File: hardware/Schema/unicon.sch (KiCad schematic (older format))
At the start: 57 parts, among them J1 PROG, J2 PWR, J3 SIDE A, J4 SIDE B, U1 LM340MP-5.0, U2 SIP21106-3.3, U3 STM32F051C8Tx, U4 AT24C16, Y1 8MHz, Y2 32768 Hz

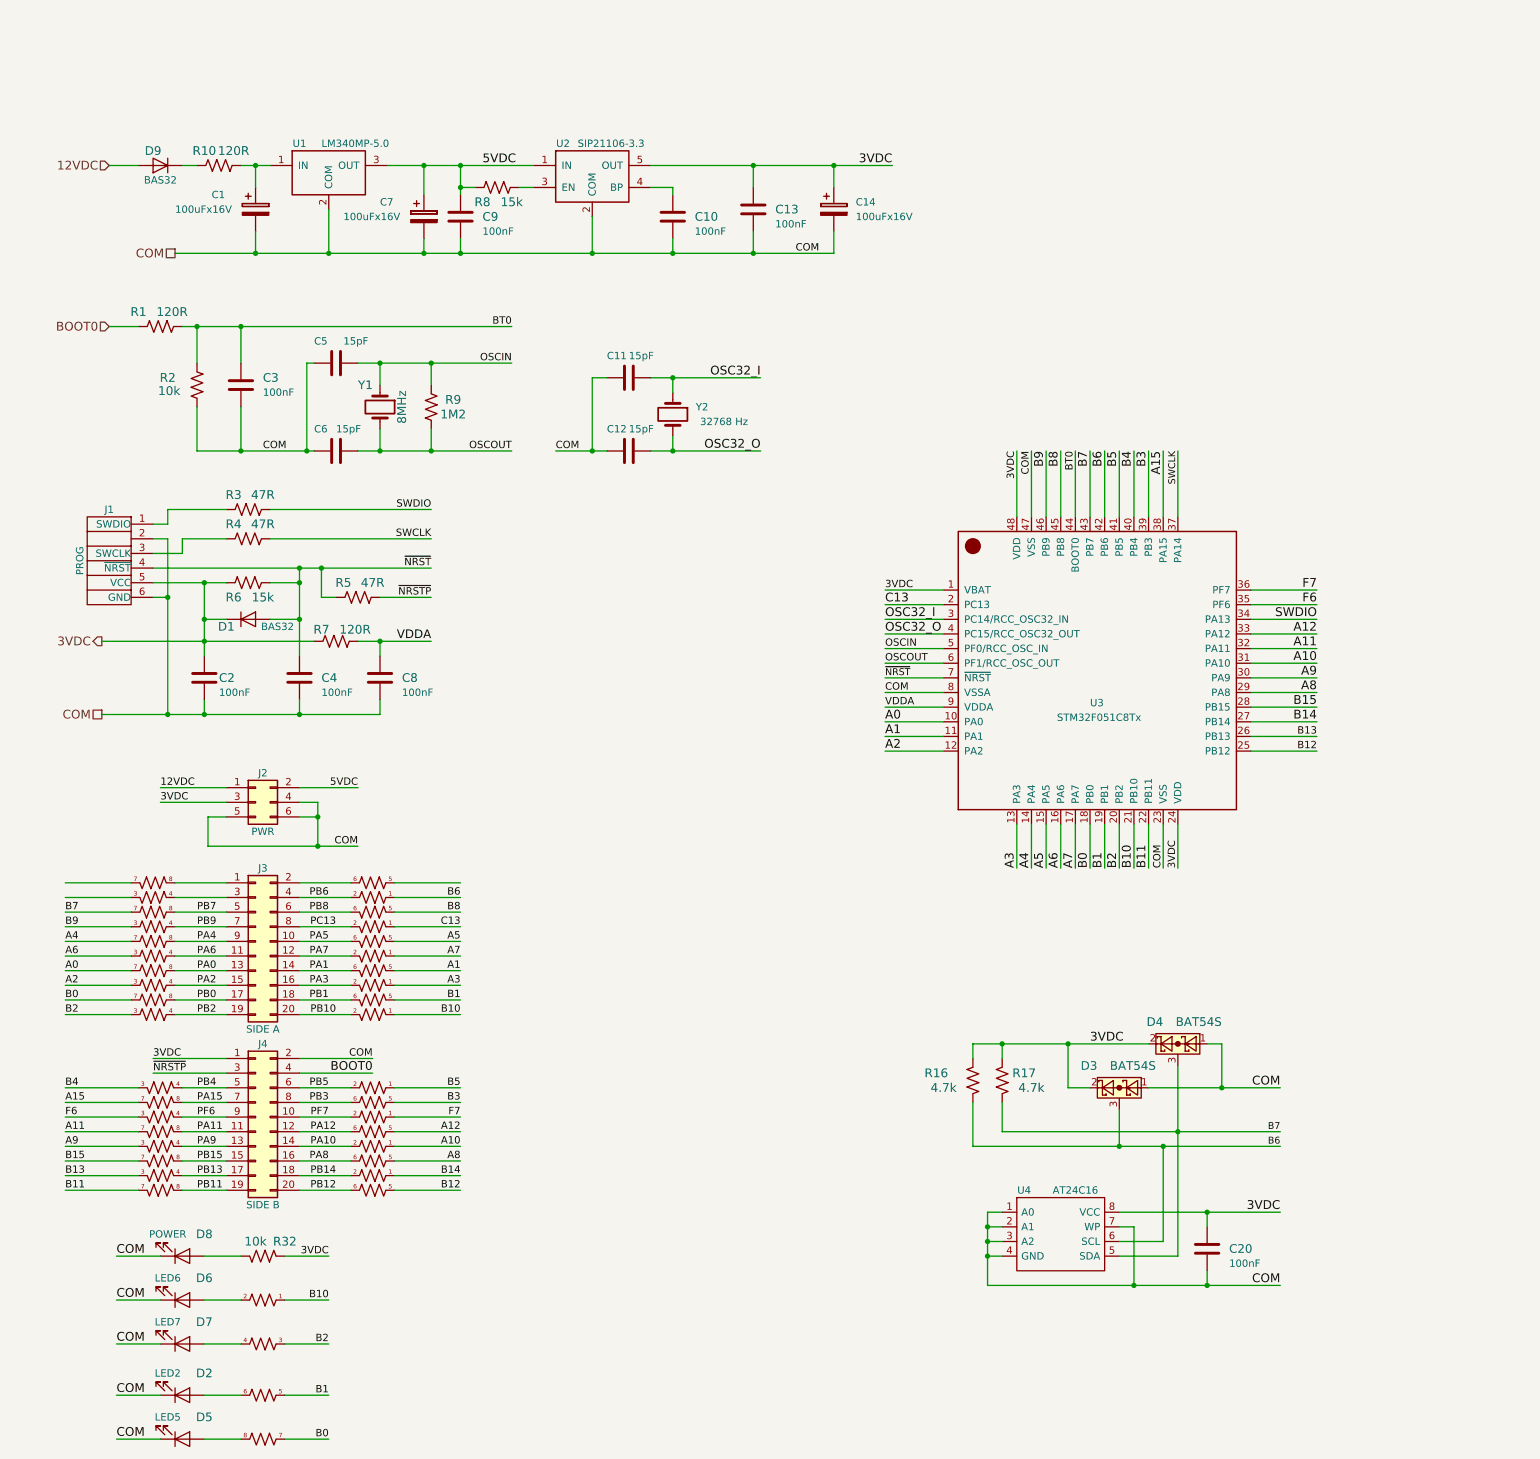
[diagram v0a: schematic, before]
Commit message: 20181012
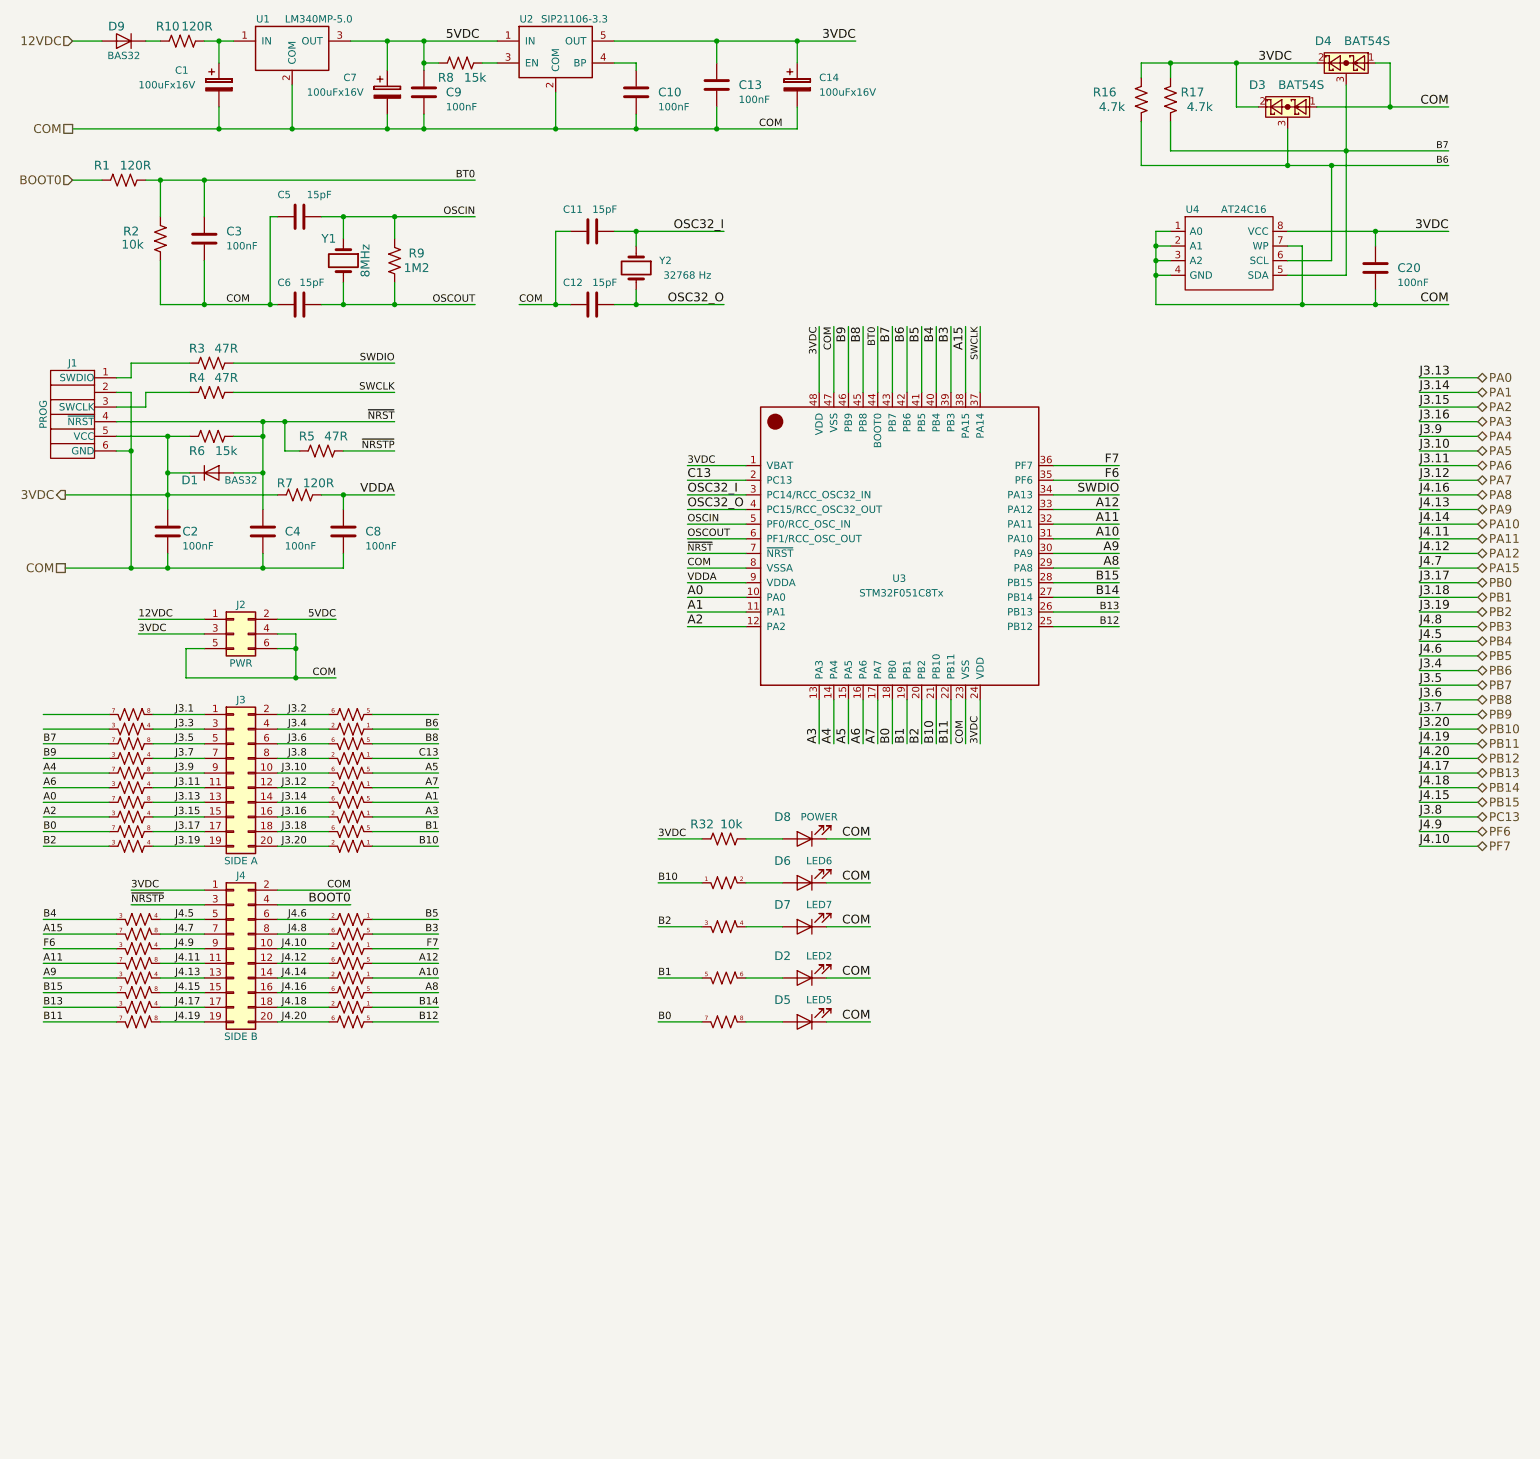
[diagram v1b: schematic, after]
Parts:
- C1, C14, C7, D2, D5, D6, D7, D8, J2, J3, J4, R10, RN1, RN14, RN2, RN3, RN4, RN5, RN6, RN7, RN8, RN9, U1, U2, U4, Y2: Sheet (none) -> mcu
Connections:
- net J3.1: now reaches J3.1 (Pin_1), RN5.8
- net J3.2: now reaches J3.2 (Pin_2), RN5.6
- net J3.3: now reaches J3.3 (Pin_3), RN5.4
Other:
- moved on the sheet: C1, C10, C11, C12, C13, C14, C2, C20, C3, C4, C5, C6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
